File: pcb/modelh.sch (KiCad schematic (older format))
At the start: 33 parts, among them J1 USB_B, J2 Conn_01x16, J3 Conn_01x08, J4 Conn_01x04, J5 AVR-ISP-6, SW1 SW_Push, U1 74HC595, U2 ATmega32U4-AU, Y1 16MHz

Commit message: PCB updates
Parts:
- removed Y1: 16MHz, Crystal:Crystal_SMD_3225-4Pin_3.2x2.5mm, symbol Device:Crystal_Small
- added Y1: Crystal_GND24, Crystal:Crystal_SMD_3225-4Pin_3.2x2.5mm, symbol Device:Crystal_GND24
- C1, C4, C6: LCSC (none) -> C15849
- C2, C3: LCSC (none) -> C1653
- C5: LCSC (none) -> C19702
- C7, C8: LCSC (none) -> C14663
- D1, D2, D3, D4, D5, D6, D7, D8: LCSC (none) -> C2128
- LED1: LCSC (none) -> C2297
- R1: LCSC (none) -> C21190
- R2: LCSC (none) -> C25804
- R3, R7: LCSC (none) -> C23345
- R4, R5, R6: LCSC (none) -> C22787
- SW1: LCSC (none) -> C318888
- U1: LCSC (none) -> C5947
- U2: LCSC (none) -> C44854
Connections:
- wire segments 135 -> 140
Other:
- moved on the sheet: C2, C3
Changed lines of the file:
@@
 F 2 "Resistor_SMD:R_0603_1608Metric" V 7480 4750 50  0001 C CNN
 F 3 "~" H 7550 4750 50  0001 C CNN
+F 4 "C22787" H 7550 4750 50  0001 C CNN "LCSC"
 	1    7550 4750
 	0    1    1    0
@@
 F 2 "Resistor_SMD:R_0603_1608Metric" V 7480 4850 50  0001 C CNN
 F 3 "~" H 7550 4850 50  0001 C CNN
+F 4 "C22787" H 7550 4850 50  0001 C CNN "LCSC"
 	1    7550 4850
 	0    1    1    0
@@
 F 2 "Resistor_SMD:R_0603_1608Metric" V 7480 5050 50  0001 C CNN
 F 3 "~" H 7550 5050 50  0001 C CNN
+F 4 "C22787" H 7550 5050 50  0001 C CNN "LCSC"
 	1    7550 5050
 	0    1    1    0
@@
 F 2 "Package_QFP:TQFP-44_10x10mm_P0.8mm" H 4850 3600 50  0001 C CIN
 F 3 "http://ww1.microchip.com/downloads/en/DeviceDoc/Atmel-7766-8-bit-AVR-ATmega16U4-32U4_Datasheet.pdf" H 4850 3600 50  0001 C CNN
+F 4 "C44854" H 4850 3600 50  0001 C CNN "LCSC"
 	1    4850 3600
 	1    0    0    -1
@@
 F 2 "Resistor_SMD:R_0603_1608Metric" V 4080 1400 50  0001 C CNN
 F 3 "~" H 4150 1400 50  0001 C CNN
+F 4 "C25804" H 4150 1400 50  0001 C CNN "LCSC"
 	1    4150 1400
 	1    0    0    -1
@@
 F 2 "Button_Switch_SMD:SW_SPST_EVPBF" H 3850 1850 50  0001 C CNN
 F 3 "~" H 3850 1850 50  0001 C CNN
+F 4 "C318888" H 3850 1650 50  0001 C CNN "LCSC"
 	1    3850 1650
 	1    0    0    -1
@@
 F 2 "Resistor_SMD:R_0603_1608Metric" V 1680 3750 50  0001 C CNN
 F 3 "~" H 1750 3750 50  0001 C CNN
+F 4 "C21190" H 1750 3750 50  0001 C CNN "LCSC"
 	1    1750 3750
 	1    0    0    -1
@@
 F 2 "LED_SMD:LED_0805_2012Metric" H 1750 4150 50  0001 C CNN
 F 3 "~" H 1750 4150 50  0001 C CNN
+F 4 "C2297" H 1750 4150 50  0001 C CNN "LCSC"
 	1    1750 4150
 	0    -1   -1   0
@@
 Wire Wire Line
 	1750 3600 1750 3500
-$Comp
-L Device:Crystal_Small Y1
-U 1 1 5ECF3F4A
-P 3900 2400
-F 0 "Y1" V 3854 2488 50  0000 L CNN
-F 1 "16MHz" V 3945 2488 50  0000 L CNN
-F 2 "Crystal:Crystal_SMD_3225-4Pin_3.2x2.5mm" H 3900 2400 50  0001 C CNN
-F 3 "~" H 3900 2400 50  0001 C CNN
-	1    3900 2400
-	0    1    1    0
-$EndComp
 Wire Wire Line
 	4250 2100 4150 2100
-Wire Wire Line
-	4250 2300 3900 2300
-Wire Wire Line
-	3900 2500 4250 2500
-$Comp
-L Device:C C2
-U 1 1 5ED22F60
-P 3650 2300
-F 0 "C2" V 3398 2300 50  0000 C CNN
-F 1 "22pF" V 3489 2300 50  0000 C CNN
-F 2 "Capacitor_SMD:C_0603_1608Metric" H 3688 2150 50  0001 C CNN
-F 3 "~" H 3650 2300 50  0001 C CNN
-	1    3650 2300
-	0    1    1    0
-$EndComp
-Wire Wire Line
-	3900 2500 3800 2500
-Connection ~ 3900 2500
-Wire Wire Line
-	3800 2300 3900 2300
-Connection ~ 3900 2300
-$Comp
-L Device:C C3
-U 1 1 5ED3A76D
-P 3650 2500
-F 0 "C3" V 3398 2500 50  0000 C CNN
-F 1 "22pF" V 3489 2500 50  0000 C CNN
-F 2 "Capacitor_SMD:C_0603_1608Metric" H 3688 2350 50  0001 C CNN
-F 3 "~" H 3650 2500 50  0001 C CNN
-	1    3650 2500
-	0    1    1    0
-$EndComp
-$Comp
-L power:GND #PWR0116
-U 1 1 5ED40F26
-P 3300 2400
-F 0 "#PWR0116" H 3300 2150 50  0001 C CNN
-F 1 "GND" H 3305 2227 50  0000 C CNN
-F 2 "" H 3300 2400 50  0001 C CNN
-F 3 "" H 3300 2400 50  0001 C CNN
-	1    3300 2400
-	0    1    1    0
-$EndComp
-Wire Wire Line
-	3500 2500 3400 2500
-Wire Wire Line
-	3400 2500 3400 2400
-Wire Wire Line
-	3400 2300 3500 2300
-Wire Wire Line
-	3300 2400 3400 2400
-Connection ~ 3400 2400
-Wire Wire Line
-	3400 2400 3400 2300
 Wire Wire Line
 	4150 1650 4150 1900
@@
 F 2 "Capacitor_SMD:C_0603_1608Metric" H 4038 2550 50  0001 C CNN
 F 3 "~" H 4000 2700 50  0001 C CNN
+F 4 "C15849" H 4000 2700 50  0001 C CNN "LCSC"
 	1    4000 2700
 	0    1    1    0
@@
 F 2 "Capacitor_SMD:C_0603_1608Metric" H 3588 3250 50  0001 C CNN
 F 3 "~" H 3550 3400 50  0001 C CNN
+F 4 "C15849" H 3550 3400 50  0001 C CNN "LCSC"
 	1    3550 3400
 	0    1    1    0
@@
 F 2 "Diode_SMD:D_SOD-323" H 2750 7000 50  0001 C CNN
 F 3 "~" H 2750 7000 50  0001 C CNN
+F 4 "C2128" H 2750 7000 50  0001 C CNN "LCSC"
 	1    2750 7000
 	1    0    0    1
@@
 F 2 "Diode_SMD:D_SOD-323" H 2750 6900 50  0001 C CNN
 F 3 "~" H 2750 6900 50  0001 C CNN
+F 4 "C2128" H 2750 6900 50  0001 C CNN "LCSC"
 	1    2750 6900
 	1    0    0    1
@@
 F 2 "Diode_SMD:D_SOD-323" H 2750 6800 50  0001 C CNN
 F 3 "~" H 2750 6800 50  0001 C CNN
+F 4 "C2128" H 2750 6800 50  0001 C CNN "LCSC"
 	1    2750 6800
 	1    0    0    1
@@
 F 2 "Diode_SMD:D_SOD-323" H 2750 6700 50  0001 C CNN
 F 3 "~" H 2750 6700 50  0001 C CNN
+F 4 "C2128" H 2750 6700 50  0001 C CNN "LCSC"
 	1    2750 6700
 	1    0    0    1
@@
 F 2 "Diode_SMD:D_SOD-323" H 2750 6600 50  0001 C CNN
 F 3 "~" H 2750 6600 50  0001 C CNN
+F 4 "C2128" H 2750 6600 50  0001 C CNN "LCSC"
 	1    2750 6600
 	1    0    0    1
@@
 F 2 "Diode_SMD:D_SOD-323" H 2750 6500 50  0001 C CNN
 F 3 "~" H 2750 6500 50  0001 C CNN
+F 4 "C2128" H 2750 6500 50  0001 C CNN "LCSC"
 	1    2750 6500
 	1    0    0    1
@@
 F 2 "Diode_SMD:D_SOD-323" H 2750 6400 50  0001 C CNN
 F 3 "~" H 2750 6400 50  0001 C CNN
+F 4 "C2128" H 2750 6400 50  0001 C CNN "LCSC"
 	1    2750 6400
 	1    0    0    1
@@
 F 2 "Diode_SMD:D_SOD-323" H 2750 6300 50  0001 C CNN
 F 3 "~" H 2750 6300 50  0001 C CNN
+F 4 "C2128" H 2750 6300 50  0001 C CNN "LCSC"
 	1    2750 6300
 	1    0    0    1
@@
 $EndComp
 $Comp
-L Device:CP C5
-U 1 1 5EF1A1A0
-P 4550 6650
-F 0 "C5" H 4668 6696 50  0000 L CNN
-F 1 "10uF" H 4668 6605 50  0000 L CNN
-F 2 "Capacitor_SMD:C_0603_1608Metric" H 4588 6500 50  0001 C CNN
-F 3 "~" H 4550 6650 50  0001 C CNN
-	1    4550 6650
-	1    0    0    -1
-$EndComp
-$Comp
 L power:+5V #PWR0106
 U 1 1 5EF21765
@@
 F 2 "Capacitor_SMD:C_0603_1608Metric" H 5038 6500 50  0001 C CNN
 F 3 "~" H 5000 6650 50  0001 C CNN
+F 4 "C15849" H 5000 6650 50  0001 C CNN "LCSC"
 	1    5000 6650
 	1    0    0    -1
@@
 F 2 "Capacitor_SMD:C_0603_1608Metric" H 5438 6500 50  0001 C CNN
 F 3 "~" H 5400 6650 50  0001 C CNN
+F 4 "C14663" H 5400 6650 50  0001 C CNN "LCSC"
 	1    5400 6650
 	1    0    0    -1
@@
 F 2 "Package_SO:SOIC-16_3.9x9.9mm_P1.27mm" H 1900 6700 50  0001 C CNN
 F 3 "http://www.ti.com/lit/ds/symlink/sn74hc595.pdf" H 1900 6700 50  0001 C CNN
+F 4 "C5947" H 1900 6700 50  0001 C CNN "LCSC"
 	1    1900 6700
 	1    0    0    -1
@@
 F 2 "Resistor_SMD:R_0603_1608Metric" V 2130 1600 50  0001 C CNN
 F 3 "~" H 2200 1600 50  0001 C CNN
+F 4 "C23345" H 2200 1600 50  0001 C CNN "LCSC"
 	1    2200 1600
 	0    -1   -1   0
@@
 F 2 "Resistor_SMD:R_0603_1608Metric" V 2130 1700 50  0001 C CNN
 F 3 "~" H 2200 1700 50  0001 C CNN
+F 4 "C23345" H 2200 1700 50  0001 C CNN "LCSC"
 	1    2200 1700
 	0    -1   -1   0
@@
 F 2 "Capacitor_SMD:C_0603_1608Metric" H 2188 5850 50  0001 C CNN
 F 3 "~" H 2150 6000 50  0001 C CNN
+F 4 "C14663" H 2150 6000 50  0001 C CNN "LCSC"
 	1    2150 6000
 	0    -1   -1   0
@@
 Wire Wire Line
 	1900 6000 1900 6100
+$Comp
+L Device:CP C5
+U 1 1 5EF1A1A0
+P 4550 6650
+F 0 "C5" H 4668 6696 50  0000 L CNN
+F 1 "10uF" H 4668 6605 50  0000 L CNN
+F 2 "Capacitor_SMD:C_0603_1608Metric" H 4588 6500 50  0001 C CNN
+F 3 "~" H 4550 6650 50  0001 C CNN
+F 4 "C19702" H 4550 6650 50  0001 C CNN "LCSC"
+	1    4550 6650
+	1    0    0    -1
+$EndComp
+$Comp
+L Device:Crystal_GND24 Y1
+U 1 1 5EF2055D
+P 3250 2400
+F 0 "Y1" V 3296 2156 50  0000 R CNN
+F 1 "Crystal_GND24" V 3400 2300 50  0000 R CNN
+F 2 "Crystal:Crystal_SMD_3225-4Pin_3.2x2.5mm" H 3250 2400 50  0001 C CNN
+F 3 "~" H 3250 2400 50  0001 C CNN
+F 4 "C13738" H 3250 2400 50  0001 C CNN "LCSC"
+	1    3250 2400
+	0    -1   -1   0
+$EndComp
+$Comp
+L power:GND #PWR0116
+U 1 1 5EF3657E
+P 3450 2400
+F 0 "#PWR0116" H 3450 2150 50  0001 C CNN
+F 1 "GND" H 3455 2227 50  0000 C CNN
+F 2 "" H 3450 2400 50  0001 C CNN
+F 3 "" H 3450 2400 50  0001 C CNN
+	1    3450 2400
+	0    -1   -1   0
+$EndComp
+Wire Wire Line
+	4250 2300 3950 2300
+Wire Wire Line
+	3950 2300 3950 2250
+Wire Wire Line
+	3950 2250 3250 2250
+Wire Wire Line
+	4250 2500 3950 2500
+Wire Wire Line
+	3950 2500 3950 2550
+Wire Wire Line
+	3950 2550 3250 2550
+$Comp
+L Device:C C2
+U 1 1 5ED22F60
+P 2900 2250
+F 0 "C2" V 2648 2250 50  0000 C CNN
+F 1 "22pF" V 2739 2250 50  0000 C CNN
+F 2 "Capacitor_SMD:C_0603_1608Metric" H 2938 2100 50  0001 C CNN
+F 3 "~" H 2900 2250 50  0001 C CNN
+F 4 "C1653" H 2900 2250 50  0001 C CNN "LCSC"
+	1    2900 2250
+	0    1    1    0
+$EndComp
+$Comp
+L Device:C C3
+U 1 1 5ED3A76D
+P 2900 2550
+F 0 "C3" V 2648 2550 50  0000 C CNN
+F 1 "22pF" V 2739 2550 50  0000 C CNN
+F 2 "Capacitor_SMD:C_0603_1608Metric" H 2938 2400 50  0001 C CNN
+F 3 "~" H 2900 2550 50  0001 C CNN
+F 4 "C1653" H 2900 2550 50  0001 C CNN "LCSC"
+	1    2900 2550
+	0    1    1    0
+$EndComp
+Wire Wire Line
+	3250 2550 3050 2550
+Connection ~ 3250 2550
+Wire Wire Line
+	3250 2250 3050 2250
+Connection ~ 3250 2250
+Wire Wire Line
+	2750 2250 2600 2250
+Wire Wire Line
+	2600 2550 2750 2550
+Wire Wire Line
+	2600 2250 2600 2400
+$Comp
+L power:GND #PWR0125
+U 1 1 5EFAE589
+P 2500 2400
+F 0 "#PWR0125" H 2500 2150 50  0001 C CNN
+F 1 "GND" H 2505 2227 50  0000 C CNN
+F 2 "" H 2500 2400 50  0001 C CNN
+F 3 "" H 2500 2400 50  0001 C CNN
+	1    2500 2400
+	0    1    1    0
+$EndComp
+Wire Wire Line
+	3050 2400 2600 2400
+Connection ~ 2600 2400
+Wire Wire Line
+	2600 2400 2600 2550
+Wire Wire Line
+	2500 2400 2600 2400
 $EndSCHEMATC

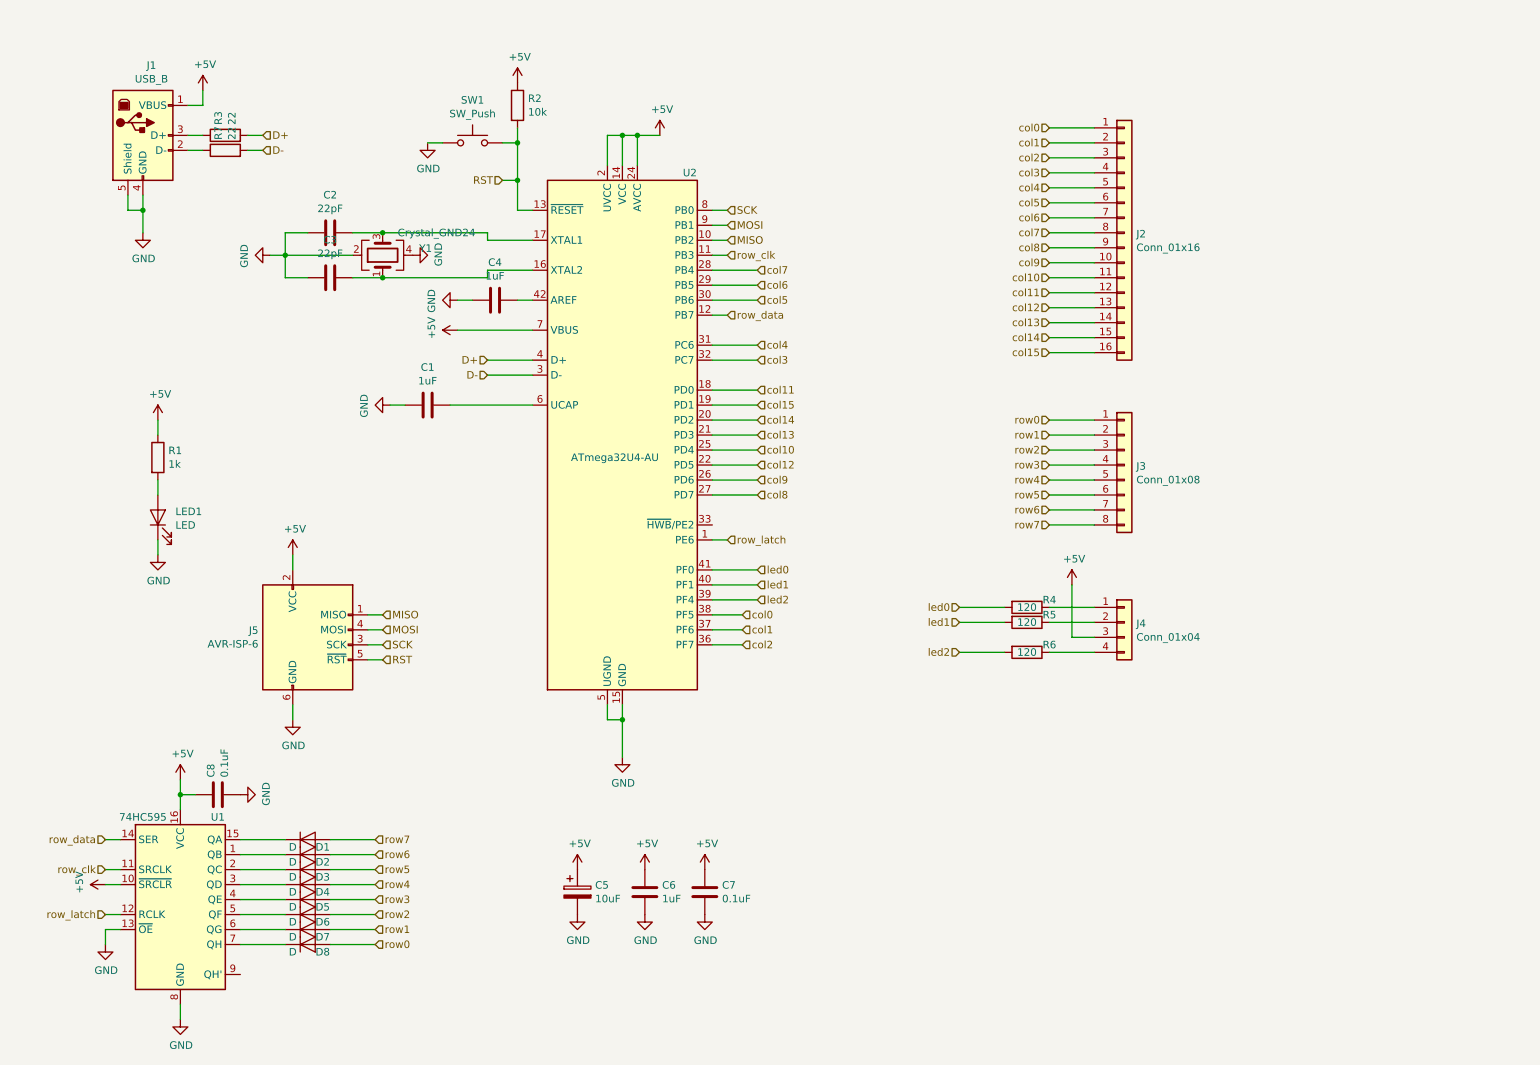
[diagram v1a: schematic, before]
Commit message: WIP
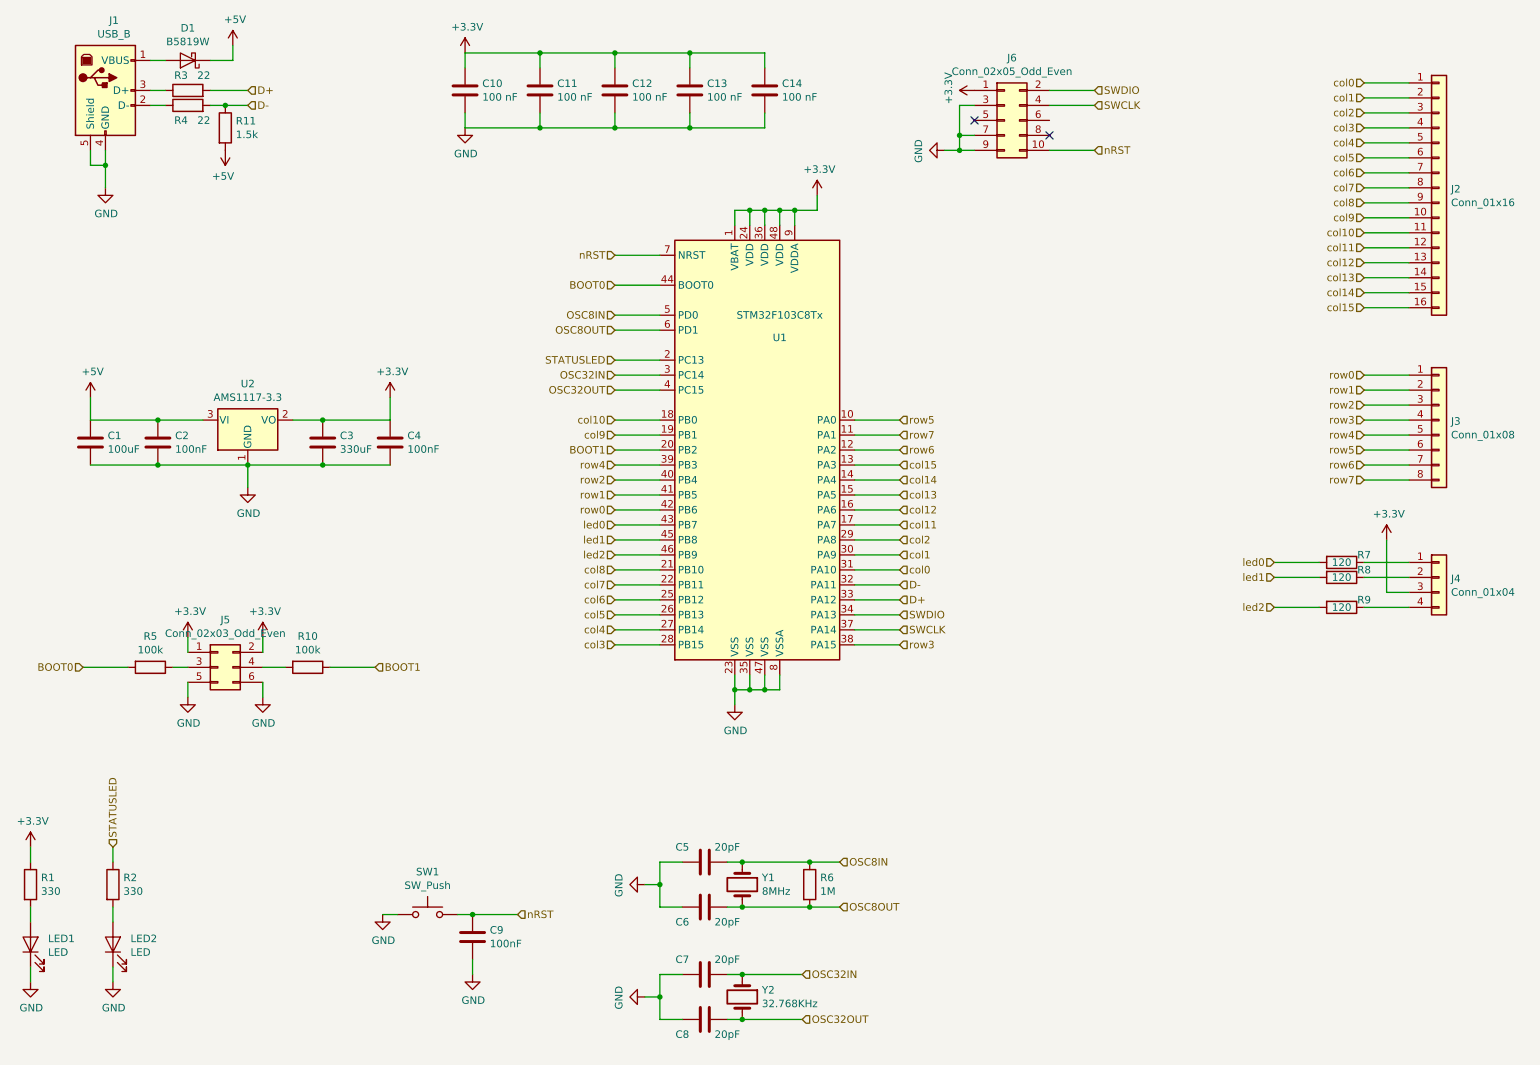
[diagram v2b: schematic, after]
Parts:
- removed C5: 10uF, Capacitor_SMD:C_0603_1608Metric, symbol Device:CP
- removed C6: 1uF, Capacitor_SMD:C_0603_1608Metric, symbol Device:C
- removed D1, D2, D3, D4, D5, D6, D7, D8: D, Diode_SMD:D_SOD-323, symbol Device:D
- removed J5: AVR-ISP-6, Connector_IDC:IDC-Header_2x03_P2.54mm_Vertical, symbol Connector:AVR-ISP-6
- removed U1: 74HC595, Package_SO:SOIC-16_3.9x9.9mm_P1.27mm, symbol 74xx:74HC595
- removed U2: ATmega32U4-AU, Package_QFP:TQFP-44_10x10mm_P0.8mm, symbol MCU_Microchip_ATmega:ATmega32U4-AU
- removed Y1: Crystal_GND24, Crystal:Crystal_SMD_3225-4Pin_3.2x2.5mm, symbol Device:Crystal_GND24
- added C10, C11, C12, C13, C14: 100 nF, Capacitor_SMD:C_0402_1005Metric, symbol Device:C
- added C2: 100nF, Capacitor_SMD:C_0402_1005Metric, symbol Device:C
- added C3: 330uF, Capacitor_SMD:C_0603_1608Metric, symbol Device:C
- added C9: 100nF, Capacitor_SMD:C_0603_1608Metric, symbol Device:C
- added D1: B5819W, Diode_SMD:D_SOD-123, symbol Device:D_Schottky
- added J5: Conn_02x03_Odd_Even, Connector_PinHeader_2.54mm:PinHeader_2x03_P2.54mm_Vertical, symbol Connector_Generic:Conn_02x03_Odd_Even
- added J6: Conn_02x05_Odd_Even, Connector_IDC:IDC-Header_2x05_P2.54mm_Vertical, symbol Connector_Generic:Conn_02x05_Odd_Even
- added LED2: LED, LED_SMD:LED_0805_2012Metric, symbol Device:LED
- added R10, R5: 100k, Resistor_SMD:R_0603_1608Metric, symbol Device:R
- added R11: 1.5k, Resistor_SMD:R_0603_1608Metric, symbol Device:R
- added R6: 1M, Resistor_SMD:R_0603_1608Metric, symbol Device:R
- added U1: STM32F103C8Tx, Package_QFP:LQFP-48_7x7mm_P0.5mm, symbol MCU_ST_STM32F1:STM32F103C8Tx
- added U2: AMS1117-3.3, Package_TO_SOT_SMD:SOT-223-3_TabPin2, symbol Regulator_Linear:AMS1117-3.3
- added Y1: 8MHz, Crystal:Crystal_SMD_5032-2Pin_5.0x3.2mm, symbol Device:Crystal
- added Y2: 32.768KHz, Crystal:Crystal_SMD_3215-2Pin_3.2x1.5mm, symbol Device:Crystal
- C1: value 1uF -> 100uF; LCSC C15849 -> (none)
- C4: value 1uF -> 100nF; footprint Capacitor_SMD:C_0603_1608Metric -> Capacitor_SMD:C_0402_1005Metric; LCSC C15849 -> (none)
- C5: renamed from C2; value 22pF -> 20pF
- C6: renamed from C3; value 22pF -> 20pF
- C7, C8: value 0.1uF -> 20pF; LCSC C14663 -> C1653
- R1: value 1k -> 330
- R2: value 10k -> 330; LCSC C25804 -> C21190
- renumbered R7 to R4, R4 to R7, R5 to R8, R6 to R9
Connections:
- net +5V: now also C1.1, C2.1, D1.1 (K), R11.2, U2.3 (VI); no longer C7.1, C8.1, J1.1 (VBUS), J4.3 (Pin_3), R1.1, R2.1
- net D+: now also U1.33 (PA12)
- net D-: now also R11.1, U1.32 (PA11)
- net GND: now also C10.2, C11.2, C12.2, C13.2, C14.2, C2.2, C3.2, C9.2, J5.5 (Pin_5), J5.6 (Pin_6), J6.3 (Pin_3), J6.7 (Pin_7), J6.9 (Pin_9), LED2.1 (K), U1.23 (VSS), U1.35 (VSS), U1.47 (VSS), U1.8 (VSSA), U2.1 (GND)
- net col0: now also U1.31 (PA10)
- net col1: now also U1.30 (PA9)
- net col10: now also U1.18 (PB0)
- net col11: now also U1.17 (PA7)
- net col12: now also U1.16 (PA6)
- net col13: now also U1.15 (PA5)
- net col14: now also U1.14 (PA4)
- net col15: now also U1.13 (PA3)
- net col2: now also U1.29 (PA8)
- net col3: now also U1.28 (PB15)
- net col4: now also U1.27 (PB14)
- net col5: now also U1.26 (PB13)
- net col6: now also U1.25 (PB12)
- net col7: now also U1.22 (PB11)
- net col8: now also U1.21 (PB10)
- net col9: now also U1.19 (PB1)
- net led0: now also U1.43 (PB7)
- net led1: now also U1.45 (PB8)
- net led2: now also U1.46 (PB9)
- net row0: now also U1.42 (PB6)
- net row1: now also U1.41 (PB5)
- net row2: now also U1.40 (PB4)
- net row3: now also U1.38 (PA15)
- net row4: now also U1.39 (PB3)
- net row5: now also U1.10 (PA0)
- net row6: now also U1.12 (PA2)
- net row7: now also U1.11 (PA1)
- net OSC8OUT: now reaches C6.1
- net OSC8OUT: now also R6.2, U1.6 (PD1), Y1.2
- net OSC8IN: now reaches C5.1
- net OSC8IN: now also R6.1, U1.5 (PD0), Y1.1
- net +3V3: now reaches C4.1
- net +3V3: now also J4.3 (Pin_3), R1.1, C10.1, C11.1, C12.1, C13.1, C14.1, C3.1, J5.1 (Pin_1), J5.2 (Pin_2), J6.1 (Pin_1), U1.1 (VBAT), U1.24 (VDD), U1.36 (VDD), U1.48 (VDD), U1.9 (VDDA), U2.2 (VO)
- net RST: no longer names the net of R2.2
- net RST: now also LED2.2 (A); no longer SW1.2
- new net: D1.2 (A), J1.1 (VBUS)
- new net: J5.4 (Pin_4), R10.2
- new net: J5.3 (Pin_3), R5.1
- new net BOOT0: R5.2, U1.44 (BOOT0)
- new net BOOT1: R10.1, U1.20 (PB2)
- new net OSC32IN: C7.1, U1.3 (PC14), Y2.1
- new net OSC32OUT: C8.1, U1.4 (PC15), Y2.2
- new net STATUSLED: R2.1, U1.2 (PC13)
- new net SWCLK: J6.4 (Pin_4), U1.37 (PA14)
- new net SWDIO: J6.2 (Pin_2), U1.34 (PA13)
- new net nRST: C9.1, J6.10 (Pin_10), SW1.2, U1.7 (NRST)
- no-connect marks 0 -> 2
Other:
- moved on the sheet: C5, C6, J1, J2, J3, J4, LED1, R1, R3, R4, R7, R8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
